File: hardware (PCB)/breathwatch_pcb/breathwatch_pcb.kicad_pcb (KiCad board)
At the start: 2 copper layers, 41.5 x 40.5 mm, 8 parts, among them J1 Conn_01x08_Socket, J2 Conn_01x08_Socket, J4 Conn_01x08_Socket, J5 USB_C_Receptacle_PowerOnly_6P, Q1 AO3401A, SW1 SW_Push

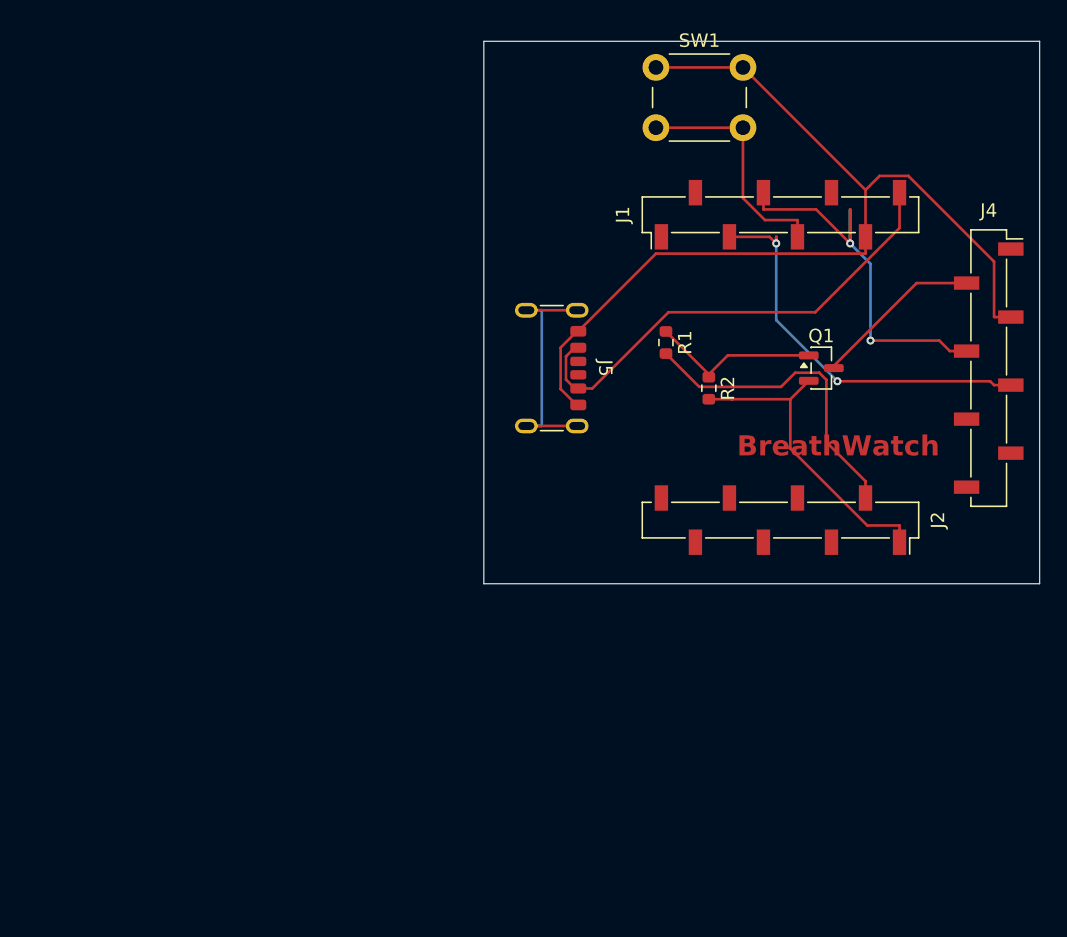
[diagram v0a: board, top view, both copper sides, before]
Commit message: PCB Design
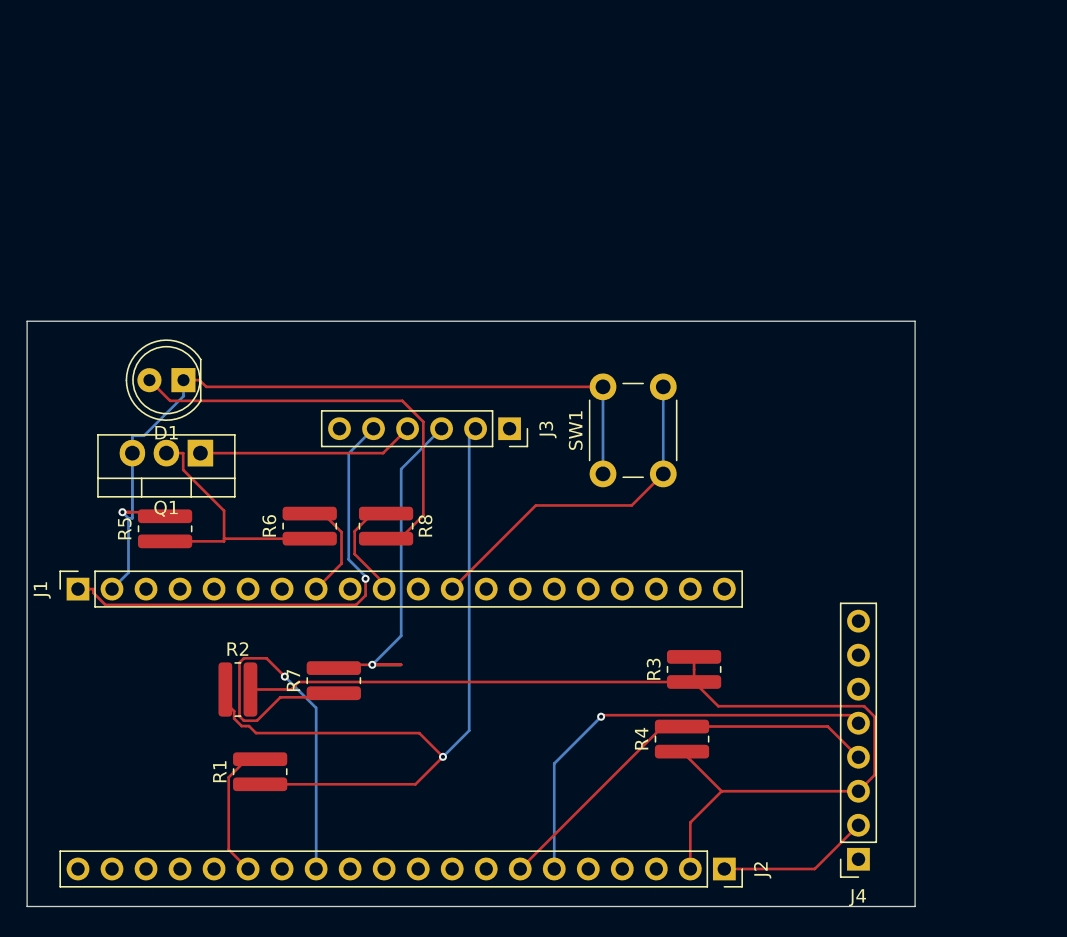
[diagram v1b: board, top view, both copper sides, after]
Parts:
- removed J5: USB_C_Receptacle_PowerOnly_6P, Connector_USB:USB_C_Receptacle_GCT_USB4125-xx-x_6P_TopMnt_Horizontal
- added D1: LED, LED_THT:LED_D5.0mm, F.Cu at (59.3, 67.8)
- added J3: Conn_01x06_Socket, Connector_PinSocket_2.54mm:PinSocket_1x06_P2.54mm_Vertical, F.Cu at (83.6, 71.4)
- added R3: 4.7k, Resistor_SMD:R_0815_2038Metric, F.Cu at (97.4, 89.4)
- added R4: 4.7k, Resistor_SMD:R_0815_2038Metric, F.Cu at (96.5, 94.6)
- added R5: 100k, Resistor_SMD:R_0815_2038Metric, F.Cu at (57.9, 78.9)
- added R6: 330, Resistor_SMD:R_0815_2038Metric, F.Cu at (68.7, 78.7)
- added R7: 4.7k, Resistor_SMD:R_0815_2038Metric, F.Cu at (70.5, 90.2)
- added R8: 330, Resistor_SMD:R_0815_2038Metric, F.Cu at (74.4, 78.7)
- J1: value Conn_01x08_Socket -> Conn_01x20_Socket; footprint Connector_PinSocket_2.54mm:PinSocket_1x08_P2.54mm_Vertical_SMD_Pin1Left -> Connector_PinSocket_2.54mm:PinSocket_1x20_P2.54mm_Vertical
- J2: value Conn_01x08_Socket -> Conn_01x20_Socket; footprint Connector_PinSocket_2.54mm:PinSocket_1x08_P2.54mm_Vertical_SMD_Pin1Right -> Connector_PinSocket_2.54mm:PinSocket_1x20_P2.54mm_Vertical
- J4: footprint Connector_PinSocket_2.54mm:PinSocket_1x08_P2.54mm_Vertical_SMD_Pin1Right -> Connector_PinSocket_2.54mm:PinSocket_1x08_P2.54mm_Vertical
- Q1: value AO3401A -> NMOS; footprint Package_TO_SOT_SMD:SOT-23 -> Package_TO_SOT_THT:TO-220-3_Vertical
- R1: value 100 -> 10k; footprint Resistor_SMD:R_0603_1608Metric -> Resistor_SMD:R_0815_2038Metric
- R2: value 100k -> 20k; footprint Resistor_SMD:R_0603_1608Metric -> Resistor_SMD:R_0815_2038Metric
- SW1: value SW_Push -> SW_Push_Dual_x2; footprint Button_Switch_THT:SW_PUSH_6mm_H7.3mm -> Button_Switch_THT:SW_PUSH_6mm_H4.3mm
- moved J1 59.4 mm to (51.4, 83.4)
- moved Q1 46.8 mm to (60.5, 73.2), turned to 180 degrees
- moved R1 44.1 mm to (65.0, 97.0), turned to 90 degrees
- moved R2 41.7 mm to (63.3, 90.9), turned to 0 degrees
- moved J4 37.9 mm to (109.7, 103.6), turned to 180 degrees
- moved SW1 30.6 mm to (90.6, 74.8), turned to 90 degrees
- moved J2 26.4 mm to (99.7, 104.3)
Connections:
- J1 pad 1: unconnected-(J1-Pin_1-Pad1) -> Net-(J1-Pin_1)
- J1 pad 2: unconnected-(J1-Pin_2-Pad2) -> Net-(D1-K)
- J1 pad 3: Net-(J1-Pin_3) -> unconnected-(J1-Pin_3-Pad3)
- J1 pad 4: Net-(J1-Pin_4) -> unconnected-(J1-Pin_4-Pad4)
- J1 pad 5: Net-(J1-Pin_5) -> unconnected-(J1-Pin_5-Pad5)
- J1 pad 7: GND -> unconnected-(J1-Pin_7-Pad7)
- J2 pad 6: unconnected-(J2-Pin_6-Pad6) -> Net-(J2-Pin_6)
- J2 pad 7: unconnected-(J2-Pin_7-Pad7) -> Net-(J2-Pin_7)
- J4 pad 2: Net-(J4-Pin_2) -> Net-(J2-Pin_1)
- J4 pad 3: GND -> Net-(J2-Pin_2)
- J4 pad 4: Net-(J1-Pin_4) -> Net-(J2-Pin_7)
- J4 pad 5: Net-(J1-Pin_3) -> Net-(J2-Pin_6)
- Q1 pad 1: Net-(Q1-G) -> Net-(J3-Pin_4)
- Q1 pad 2: Net-(J2-Pin_1) -> Net-(Q1-G)
- Q1 pad 3: Net-(J4-Pin_2) -> Net-(D1-K)
- R1 pad 1: Net-(Q1-G) -> Net-(J3-Pin_2)
- R1 pad 2: Net-(J2-Pin_2) -> Net-(J2-Pin_15)
- R2 pad 1: Net-(Q1-G) -> Net-(J3-Pin_2)
- R2 pad 2: Net-(J2-Pin_1) -> Net-(J2-Pin_2)
- SW1 pad 1: GND -> Net-(D1-K)
- SW1 pad 2: Net-(J1-Pin_5) -> Net-(J1-Pin_12)
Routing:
- net GND: track 72.8 -> 0.00 mm
- net Net-(D1-K): track 0.00 -> 63.1 mm, vias 0 -> 1
- net Net-(J3-Pin_2): track 0.00 -> 59.2 mm, vias 0 -> 1
- net Net-(J2-Pin_2): track 23.7 -> 77.0 mm
- net Net-(J1-Pin_1): track 0.00 -> 36.2 mm, vias 0 -> 1
- net Net-(J1-Pin_4): track 34.3 -> 0.00 mm, vias 2 -> 0
- net Net-(J2-Pin_6): track 0.00 -> 33.0 mm, vias 0 -> 1
- net Net-(D1-A): track 0.00 -> 32.2 mm
- net Net-(J2-Pin_13): track 0.00 -> 31.4 mm, vias 0 -> 1
- net Net-(J3-Pin_3): track 0.00 -> 31.4 mm, vias 0 -> 1
- net Net-(J1-Pin_3): track 30.9 -> 0.00 mm, vias 2 -> 0
- net Net-(J2-Pin_7): track 0.00 -> 30.6 mm
- net Net-(J1-Pin_8): track 35.7 -> 7.99 mm
- net Net-(J1-Pin_12): track 0.00 -> 25.8 mm
- net unconnected-(J5-SHIELD-PadS1): track 18.5 -> 0.00 mm
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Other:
- board size 41.5 x 40.5 mm -> 66.3 x 43.7 mm
- board text removed: "BreathWatch"
